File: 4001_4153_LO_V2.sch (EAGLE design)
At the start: 112 parts, among them IC1 74LVC2G17GV,125, IC10 MCP6H01, IC2 74LVC2G17GV,125, IC3 74LVC2G17GV,125, IC4 ADF4001BRUZ, IC5 ATTINY45V-10SU, IC6 7805DT, IC7 7809DT, IC8 LD1117AS33TR, IC9 ADF4153BRUZ-RL7, Q1 PGA105+

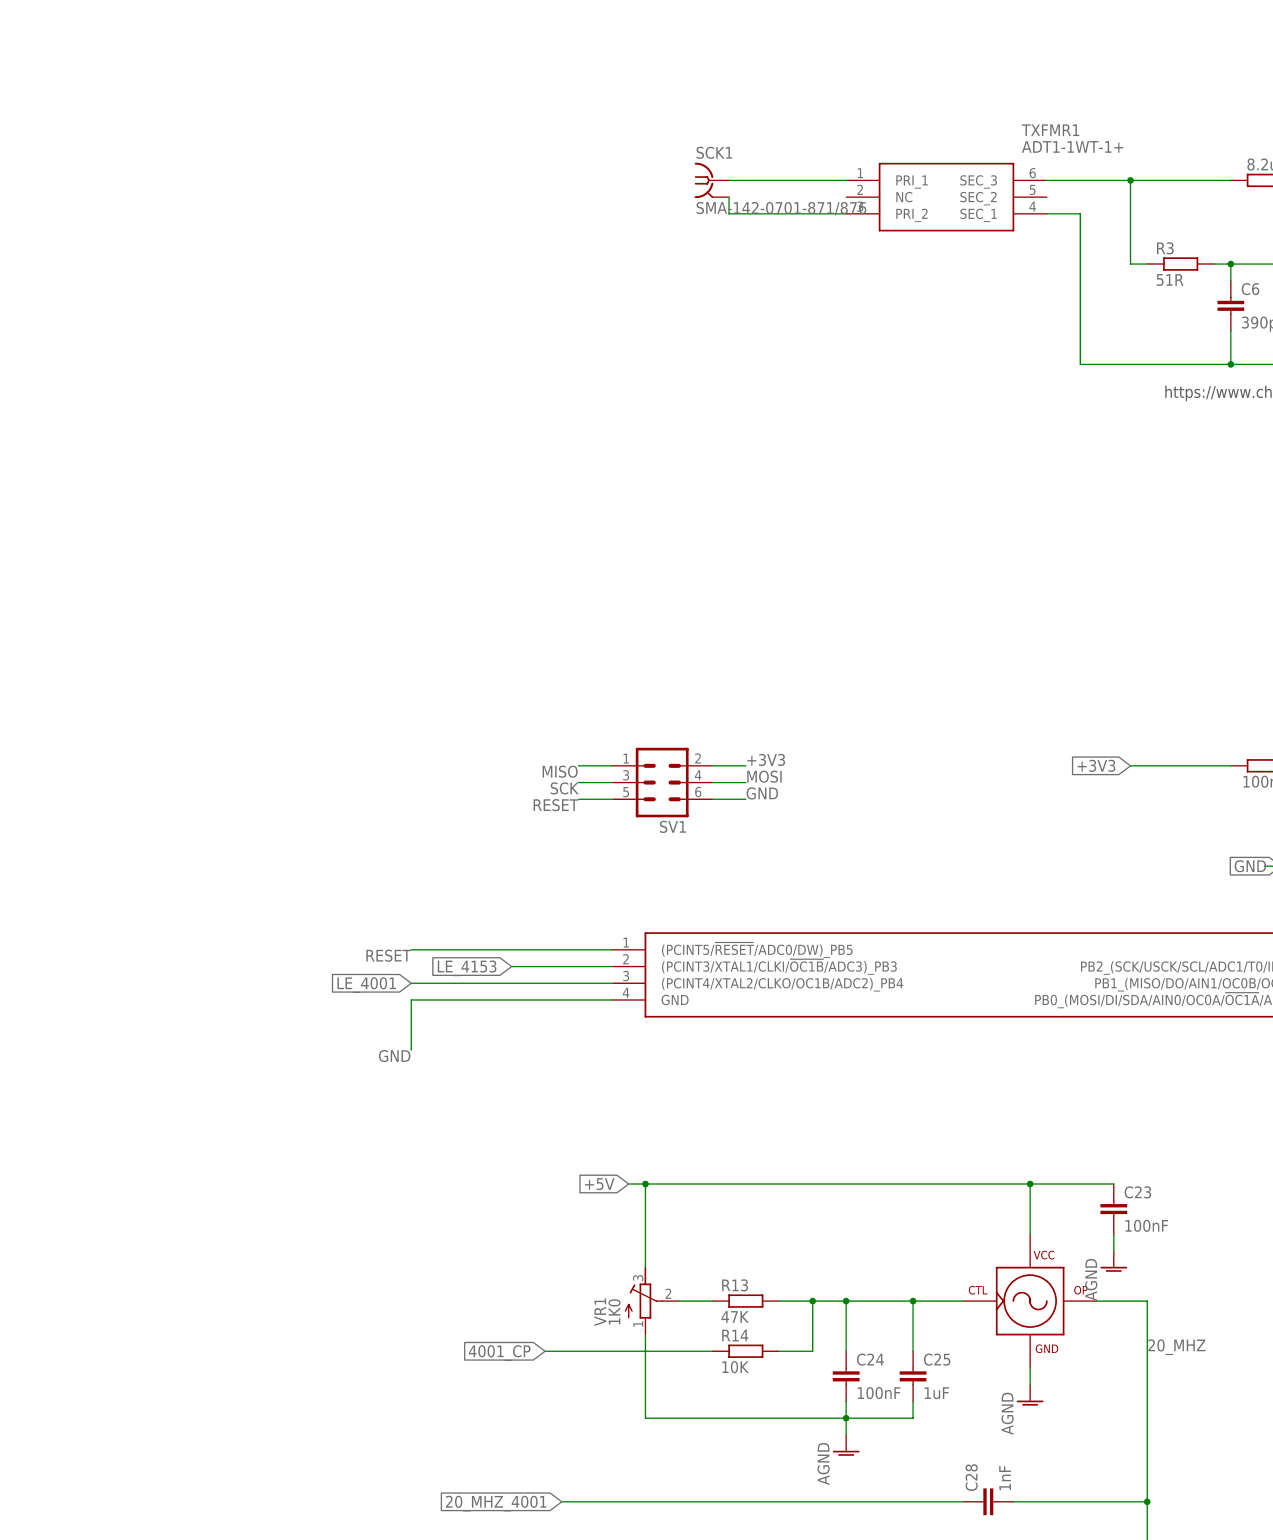
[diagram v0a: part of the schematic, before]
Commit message: JLC release
As issued to JLC
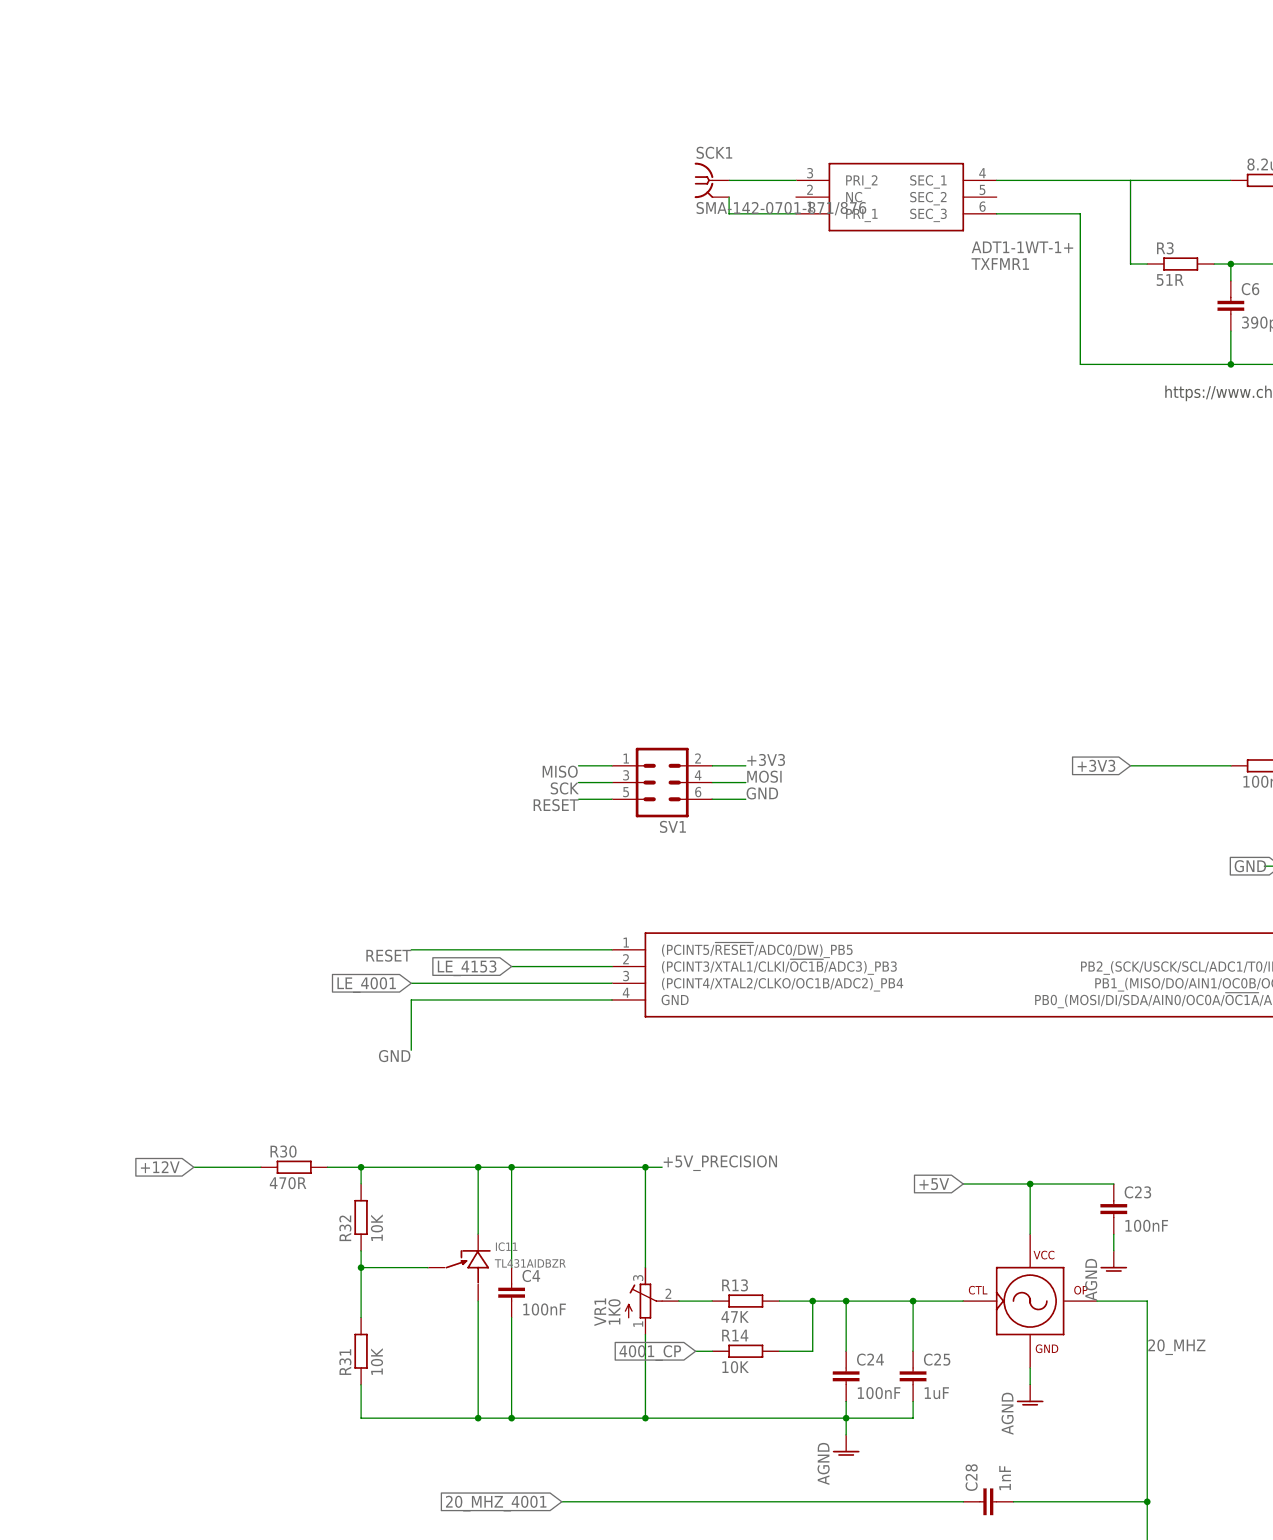
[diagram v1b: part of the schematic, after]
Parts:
- added C4: 100nF, rcl:C-EUC0603
- added IC11: TL431AIDBZR, RF:TL431AIDBZR
- added R30: 470R, rcl:R-EU_R0603
- added R31, R32: 10K, rcl:R-EU_R0603
- IC10: value MCP6H01 -> MCP6H01T-E/LT; MPN (none) -> MCP6H01T-E/LT; OC_FARNELL (none) -> 2920751
- SV1: MPN (none) -> MC-254-06-00-ST-DIP; OC_FARNELL (none) -> 2843525
- VR1: MPN (none) -> 3296Y-1-103LF; OC_FARNELL (none) -> 9353186
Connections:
- new net +5V_PRECISION: C4.1, IC11.CATHODE, R30.2, R32.2, VR1.A
- new net N$42: IC11.CTRL, R31.2, R32.1
- net +12V: now also R30.1
- net +5V: no longer VR1.A
- net GND: now also C4.2, IC11.ANODE, R31.1, TXFMR1.PRI_1, TXFMR1.SEC_3; no longer TXFMR1.PRI_2, TXFMR1.SEC_1
- net N$33: now also TXFMR1.SEC_1; no longer TXFMR1.SEC_3
- net N$34: now also TXFMR1.PRI_2; no longer TXFMR1.PRI_1
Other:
- moved on the sheet: TXFMR1
